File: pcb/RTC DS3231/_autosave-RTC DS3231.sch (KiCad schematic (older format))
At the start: 22 parts, among them J101 Conn_01x06_Male, J102 Conn_01x04_Male, U101 DS3231M, U102 AT24CS32-SSHM

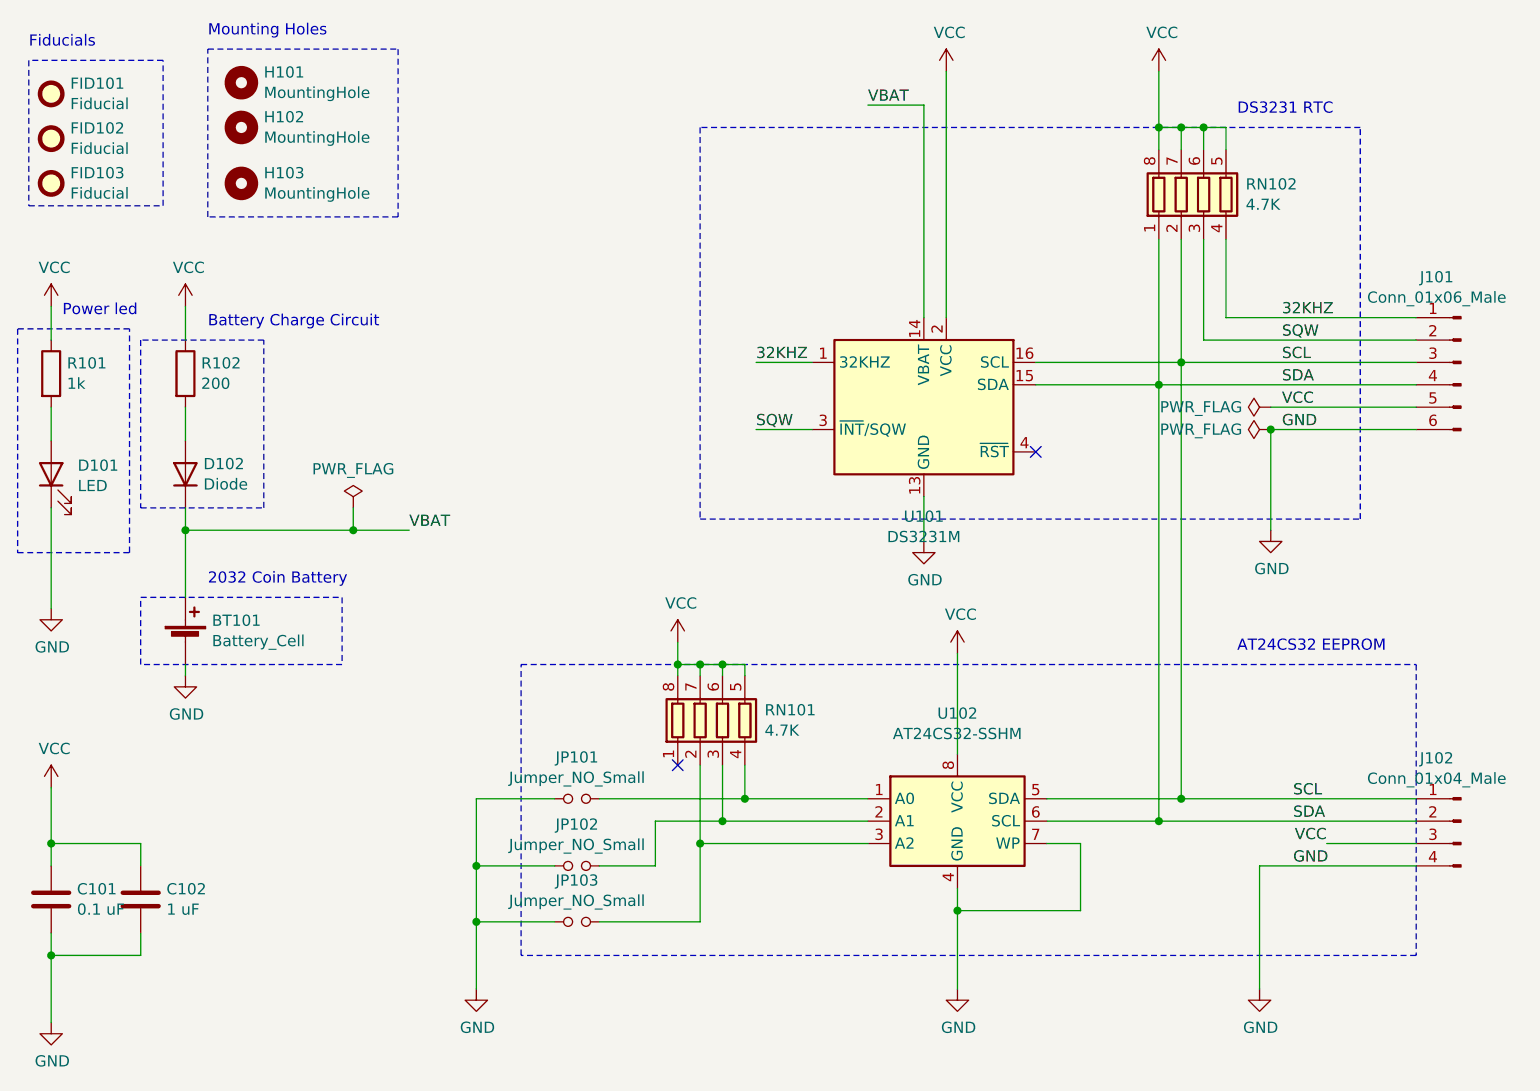
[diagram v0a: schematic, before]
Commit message: Ruteos PCB.
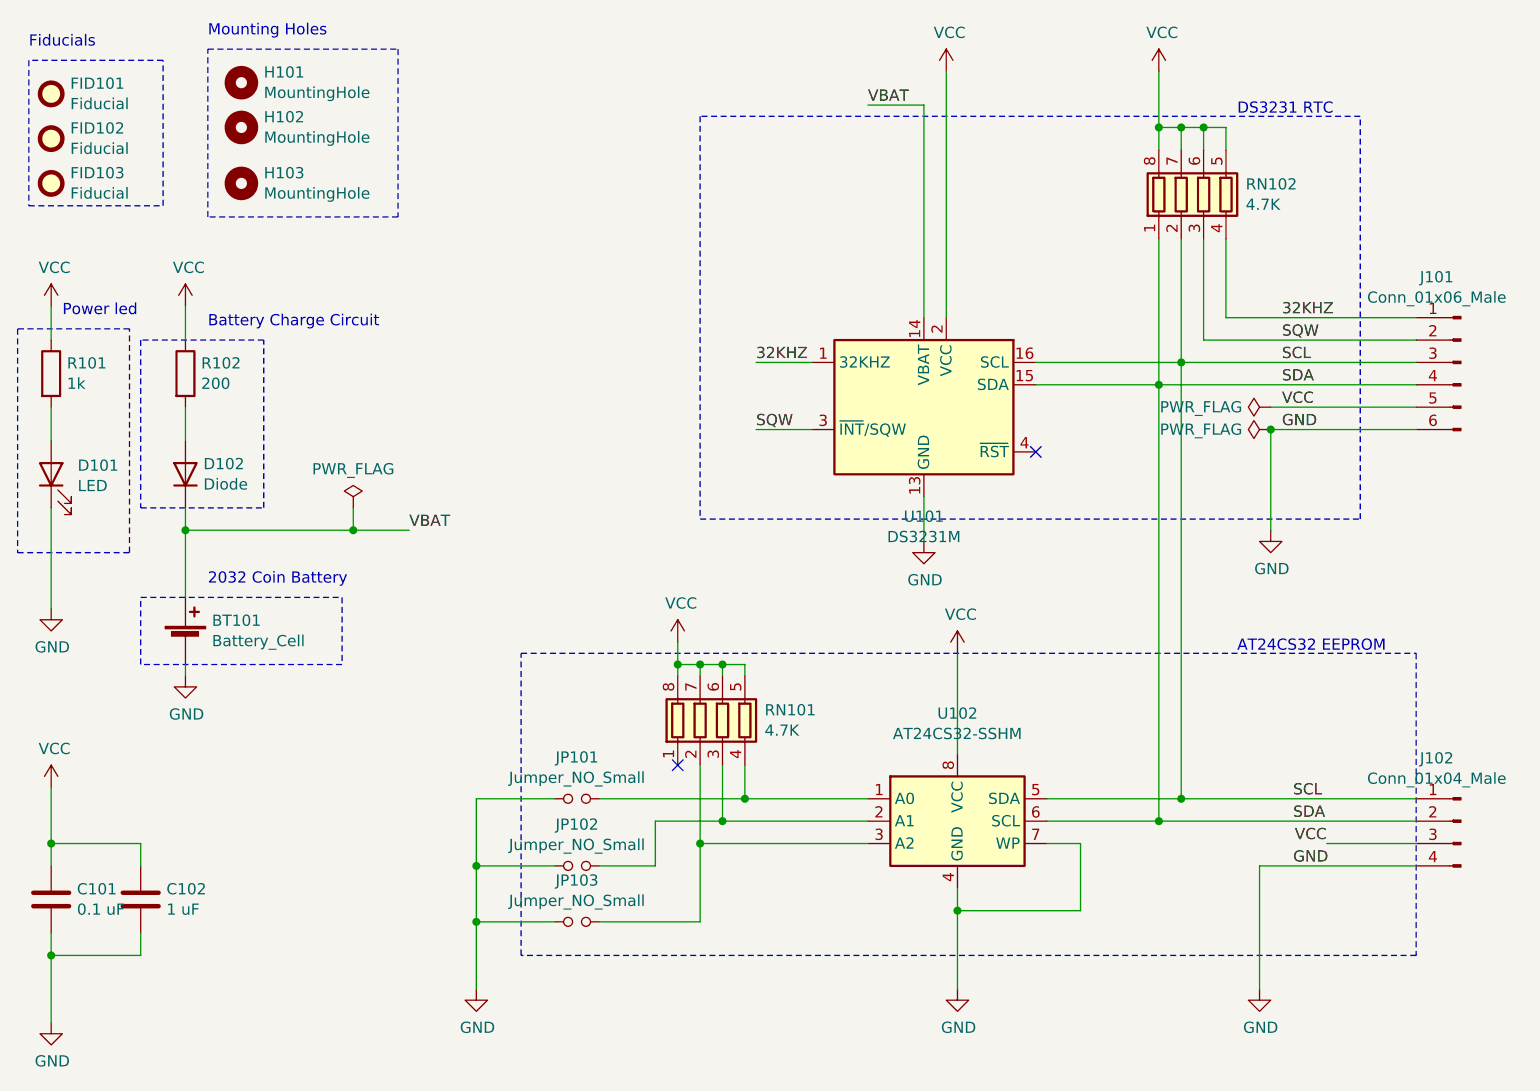
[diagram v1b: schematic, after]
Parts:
- JP101, JP102, JP103: footprint TestPoint:TestPoint_2Pads_Pitch2.54mm_Drill0.8mm -> Jumper:SolderJumper-2_P1.3mm_Open_Pad1.0x1.5mm
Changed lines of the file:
@@
 F 0 "JP101" H 5000 4835 50  0000 C CNN
 F 1 "Jumper_NO_Small" H 5000 4744 50  0000 C CNN
-F 2 "TestPoint:TestPoint_2Pads_Pitch2.54mm_Drill0.8mm" H 5000 4650 50  0001 C CNN
+F 2 "Jumper:SolderJumper-2_P1.3mm_Open_Pad1.0x1.5mm" H 5000 4650 50  0001 C CNN
 F 3 "~" H 5000 4650 50  0001 C CNN
 	1    5000 4650
@@
 F 0 "JP102" H 5000 5135 50  0000 C CNN
 F 1 "Jumper_NO_Small" H 5000 5044 50  0000 C CNN
-F 2 "TestPoint:TestPoint_2Pads_Pitch2.54mm_Drill0.8mm" H 5000 4950 50  0001 C CNN
+F 2 "Jumper:SolderJumper-2_P1.3mm_Open_Pad1.0x1.5mm" H 5000 4950 50  0001 C CNN
 F 3 "~" H 5000 4950 50  0001 C CNN
 	1    5000 4950
@@
 F 0 "JP103" H 5000 5385 50  0000 C CNN
 F 1 "Jumper_NO_Small" H 5000 5294 50  0000 C CNN
-F 2 "TestPoint:TestPoint_2Pads_Pitch2.54mm_Drill0.8mm" H 5000 5200 50  0001 C CNN
+F 2 "Jumper:SolderJumper-2_P1.3mm_Open_Pad1.0x1.5mm" H 5000 5200 50  0001 C CNN
 F 3 "~" H 5000 5200 50  0001 C CNN
 	1    5000 5200
@@
 	5550 3400 8500 3400
 Wire Notes Line
-	8500 3400 8500 1650
-Wire Notes Line
-	8500 1650 5550 1650
-Wire Notes Line
-	5550 1650 5550 3400
+	8500 3400 8500 1600
+Wire Notes Line
+	8500 1600 5550 1600
+Wire Notes Line
+	5550 1600 5550 3400
 Text Notes 7950 1600 0    50   ~ 0
 DS3231 RTC
 Wire Notes Line
-	4750 4050 8750 4050
-Wire Notes Line
-	8750 4050 8750 5350
+	4750 4000 8750 4000
+Wire Notes Line
+	8750 4000 8750 5350
 Wire Notes Line
 	8750 5350 4750 5350
 Wire Notes Line
-	4750 5350 4750 4050
+	4750 5350 4750 4000
 Text Notes 7950 4000 0    50   ~ 0
 AT24CS32 EEPROM
